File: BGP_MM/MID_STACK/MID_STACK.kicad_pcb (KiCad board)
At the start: 2 copper layers, 20 x 26 mm, 7 parts, among them P1 CONN_01X04, P2 CONN_01X09

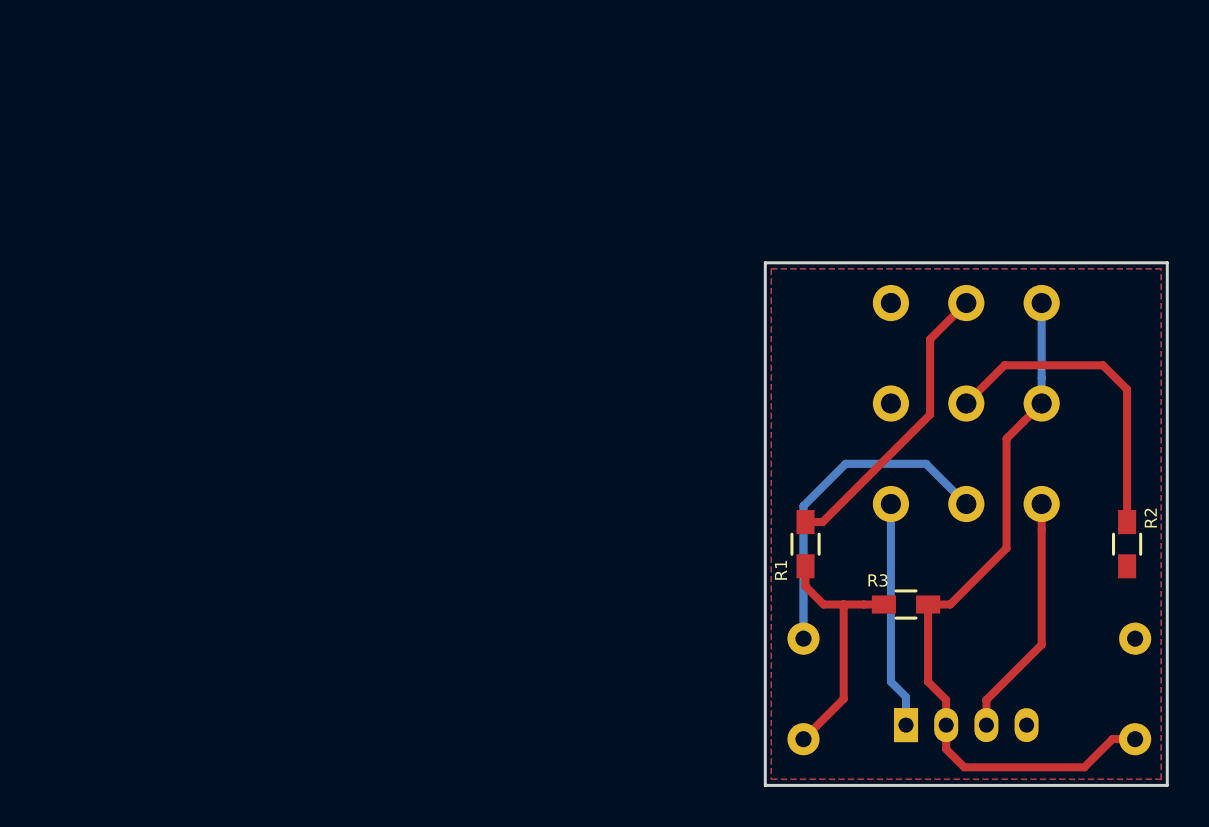
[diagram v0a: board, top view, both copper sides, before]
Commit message: MM Finished board layouts
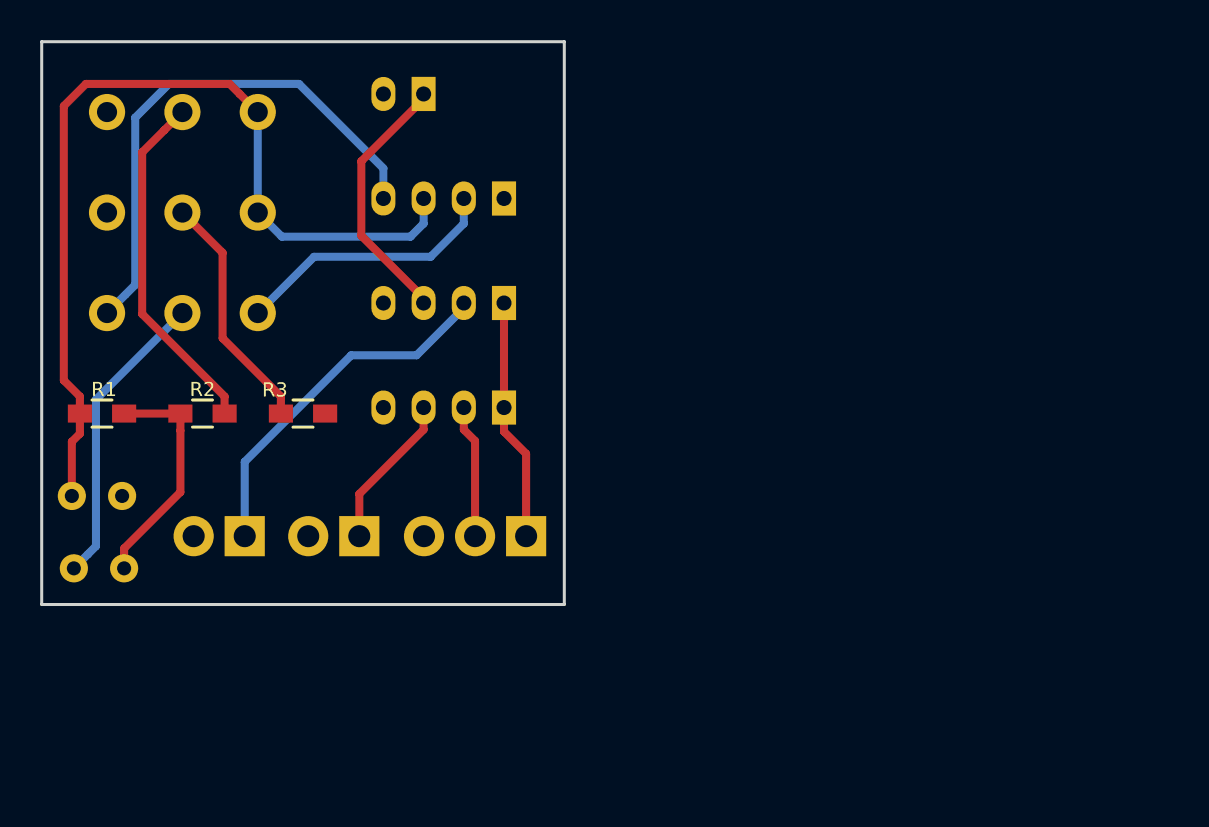
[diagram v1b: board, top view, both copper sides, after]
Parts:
- added J1: Conn_01x04_Male, Connectors_JST:JST_PH_B4B-PH-K_04x2.00mm_Straight, B.Cu at (152.0, 88.8)
- added J2: Conn_01x02_Male, Connectors_JST:JST_PH_B2B-PH-K_02x2.00mm_Straight, B.Cu at (148.0, 83.6)
- added J3: Conn_01x04_Male, Connectors_JST:JST_PH_B4B-PH-K_04x2.00mm_Straight, B.Cu at (152.0, 99.2)
- added J4: Conn_01x04_Male, Connectors_JST:JST_PH_B4B-PH-K_04x2.00mm_Straight, B.Cu at (152.0, 94.0)
- added P3: CONN_01X02, Terminal_Blocks:TerminalBlock_Pheonix_MPT-2.54mm_2pol, B.Cu at (144.8, 105.6)
- added P4: CONN_01X03, Terminal_Blocks:TerminalBlock_Pheonix_MPT-2.54mm_3pol, B.Cu at (153.1, 105.6)
- C1, C2: footprint Capacitor_THT:C_Rect_L7.2mm_W2.5mm_P5.00mm_FKS2_FKP2_MKS2_MKP2 -> Capacitor_THT:C_Rect_L4.6mm_W3.0mm_P2.50mm_MKS02_FKP02
- P1: value CONN_01X04 -> CONN_01X09; footprint Connectors_JST:JST_PH_B4B-PH-K_04x2.00mm_Straight -> LIBS:Potentiometer_Alpha_Tripple_Vertical_Dual_Shaft
- P2: value CONN_01X09 -> CONN_01X02; footprint LIBS:Potentiometer_Alpha_Tripple_Vertical_Dual_Shaft -> Terminal_Blocks:TerminalBlock_Pheonix_MPT-2.54mm_2pol
- R1: value 4.7k -> 200k
- R2: value 4.7k -> 10k
- R3: value 100k -> 10k
- moved C2 54.3 mm to (130.5, 103.6), turned to 0 degrees
- moved P1 50.1 mm to (132.2, 84.5), turned to 90 degrees
- moved R2 46.5 mm to (137.0, 99.5), turned to 0 degrees
- moved C1 36.5 mm to (130.6, 107.2), turned to 0 degrees
- moved R1 35.6 mm to (132.0, 99.5), turned to 180 degrees
- moved P2 34.2 mm to (139.1, 105.6), turned to 180 degrees
- moved R3 31.5 mm to (142.0, 99.5)
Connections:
- C2 pad 1: /F1_1 -> /MID_R
- P1 pad 1: /MID_I -> Net-(P1-Pad1)
- P1 pad 2: /F1_1 -> /F1_2
- P1 pad 3: /MID_O -> /MID_R
- P1 pad 4: /Vref -> Net-(P1-Pad4)
- P2 pad 1: Net-(P2-Pad1) -> /JZ_I
- P2 pad 2: /F1_2 -> Earth
- R1 pad 2: /F1_2 -> /MID_R
- R2 pad 1: /F2_2 -> Net-(C1-Pad2)
- R2 pad 2: /Vref -> /F1_2
- R3 pad 1: Net-(C1-Pad2) -> /F2_2
- R3 pad 2: /F1_1 -> /Vref
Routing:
- net /MID_R: track 0.00 -> 45.8 mm
- net /F1_1: track 36.3 -> 0.00 mm
- net /JZ_I: track 0.00 -> 18.0 mm
- net /MID_I: track 11.4 -> 26.6 mm
- net /SIG_O: track 0.00 -> 13.0 mm
- net /MM_BH: track 0.00 -> 12.1 mm
- net /MM_NH: track 0.00 -> 7.73 mm
- net /MM_BC: track 0.00 -> 6.63 mm
- net /F2_2: track 15.9 -> 12.0 mm
- net /F1_2: track 14.7 -> 17.5 mm
- net /VOL2: track 16.4 -> 14.9 mm
- net /MID_O: track 12.1 -> 13.3 mm
- net Net-(C1-Pad2): track 12.8 -> 11.7 mm
- added copper zone on B.Cu, net Earth
- removed copper zone on B.Cu, net (none)
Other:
- board size 20 x 26 mm -> 26 x 28 mm
